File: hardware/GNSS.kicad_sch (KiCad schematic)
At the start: 14 parts, among them J1 Conn_Coaxial, Q1 PMOS, Q2 NMOS, U5 LT6003HDC-TRMPBF, U6 NC7WZ07P6X, U7 NC7WZ07P6X

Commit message: Changes from Reddit review 1
Changed connector, impedance matched the RF traces, changed board to square
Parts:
- J1: footprint Connector_Coaxial:U.FL_Molex_MCRF_73412-0110_Vertical -> Connector_Coaxial:SMA_BAT_Wireless_BWSMA-KWE-Z001
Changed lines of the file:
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@@
 			)
 		)
-		(property "Footprint" "Connector_Coaxial:U.FL_Molex_MCRF_73412-0110_Vertical"
+		(property "Footprint" "Connector_Coaxial:SMA_BAT_Wireless_BWSMA-KWE-Z001"
 			(at 44.45 27.94 0)
 			(effects

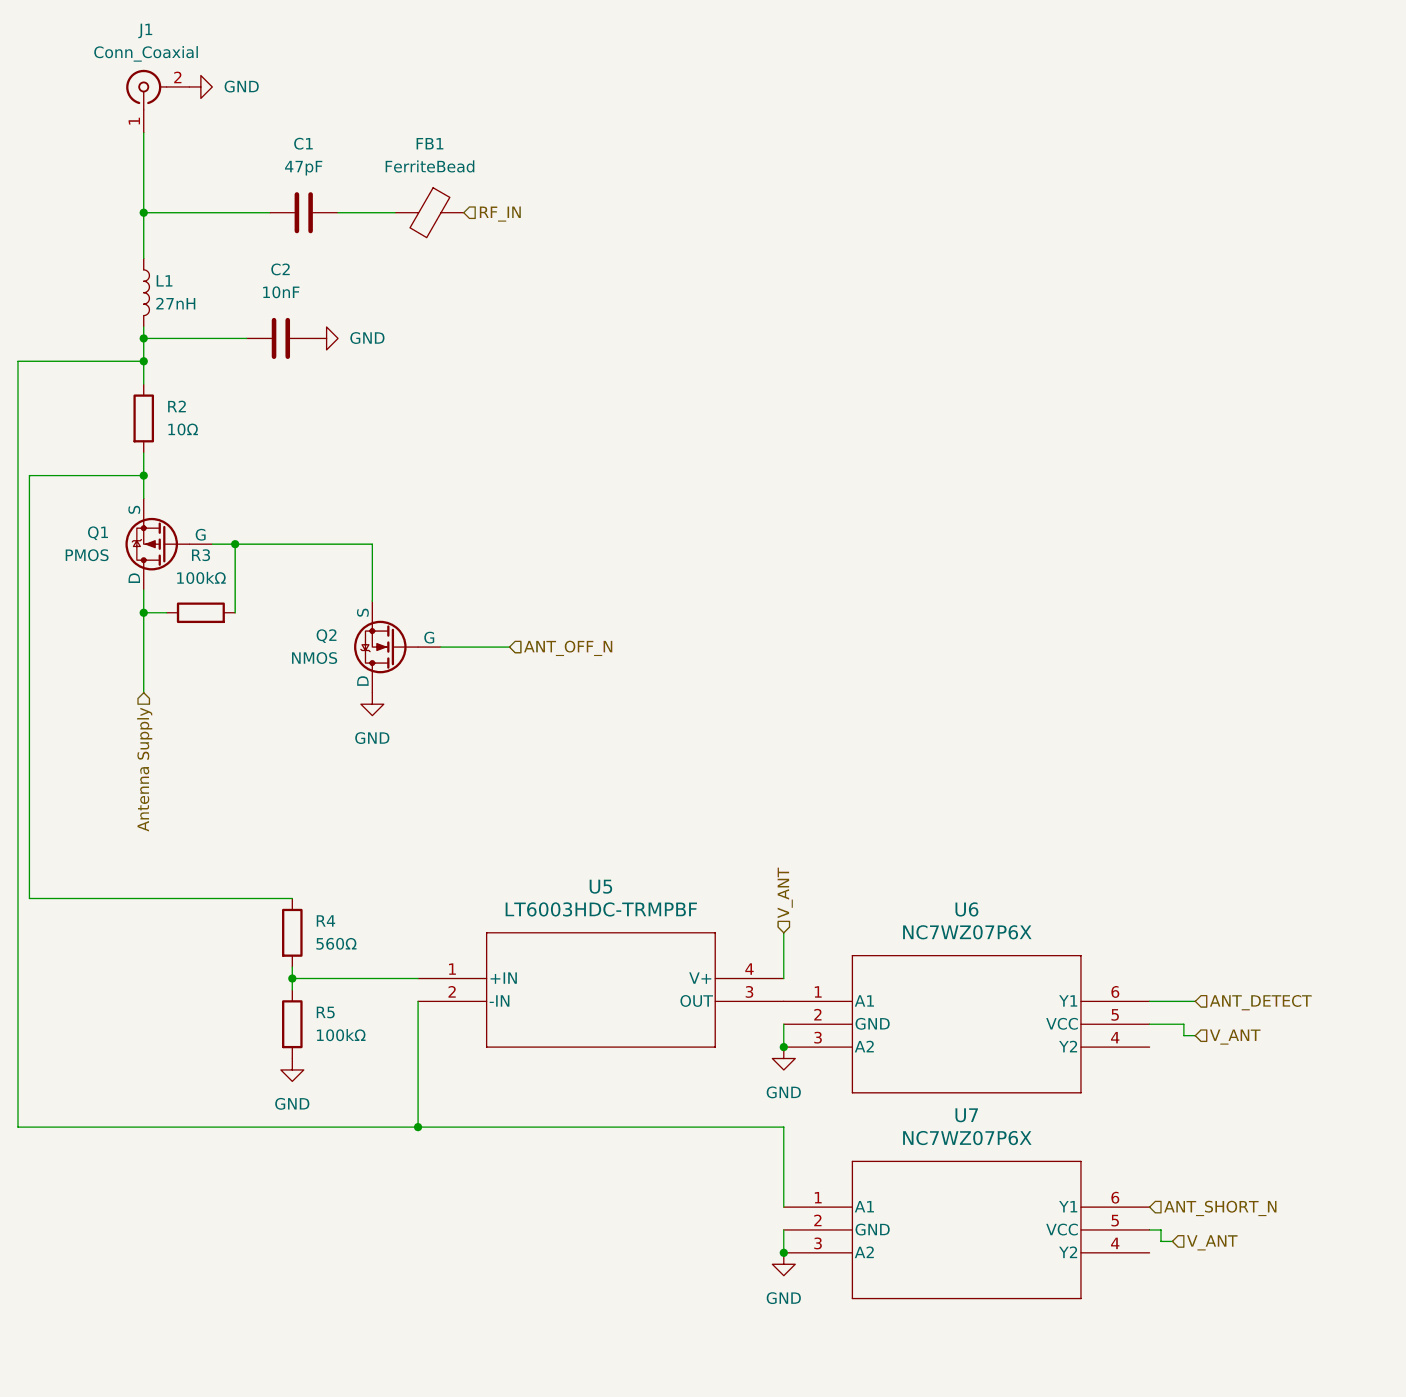
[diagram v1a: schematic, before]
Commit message: many fatal fuck-ups found
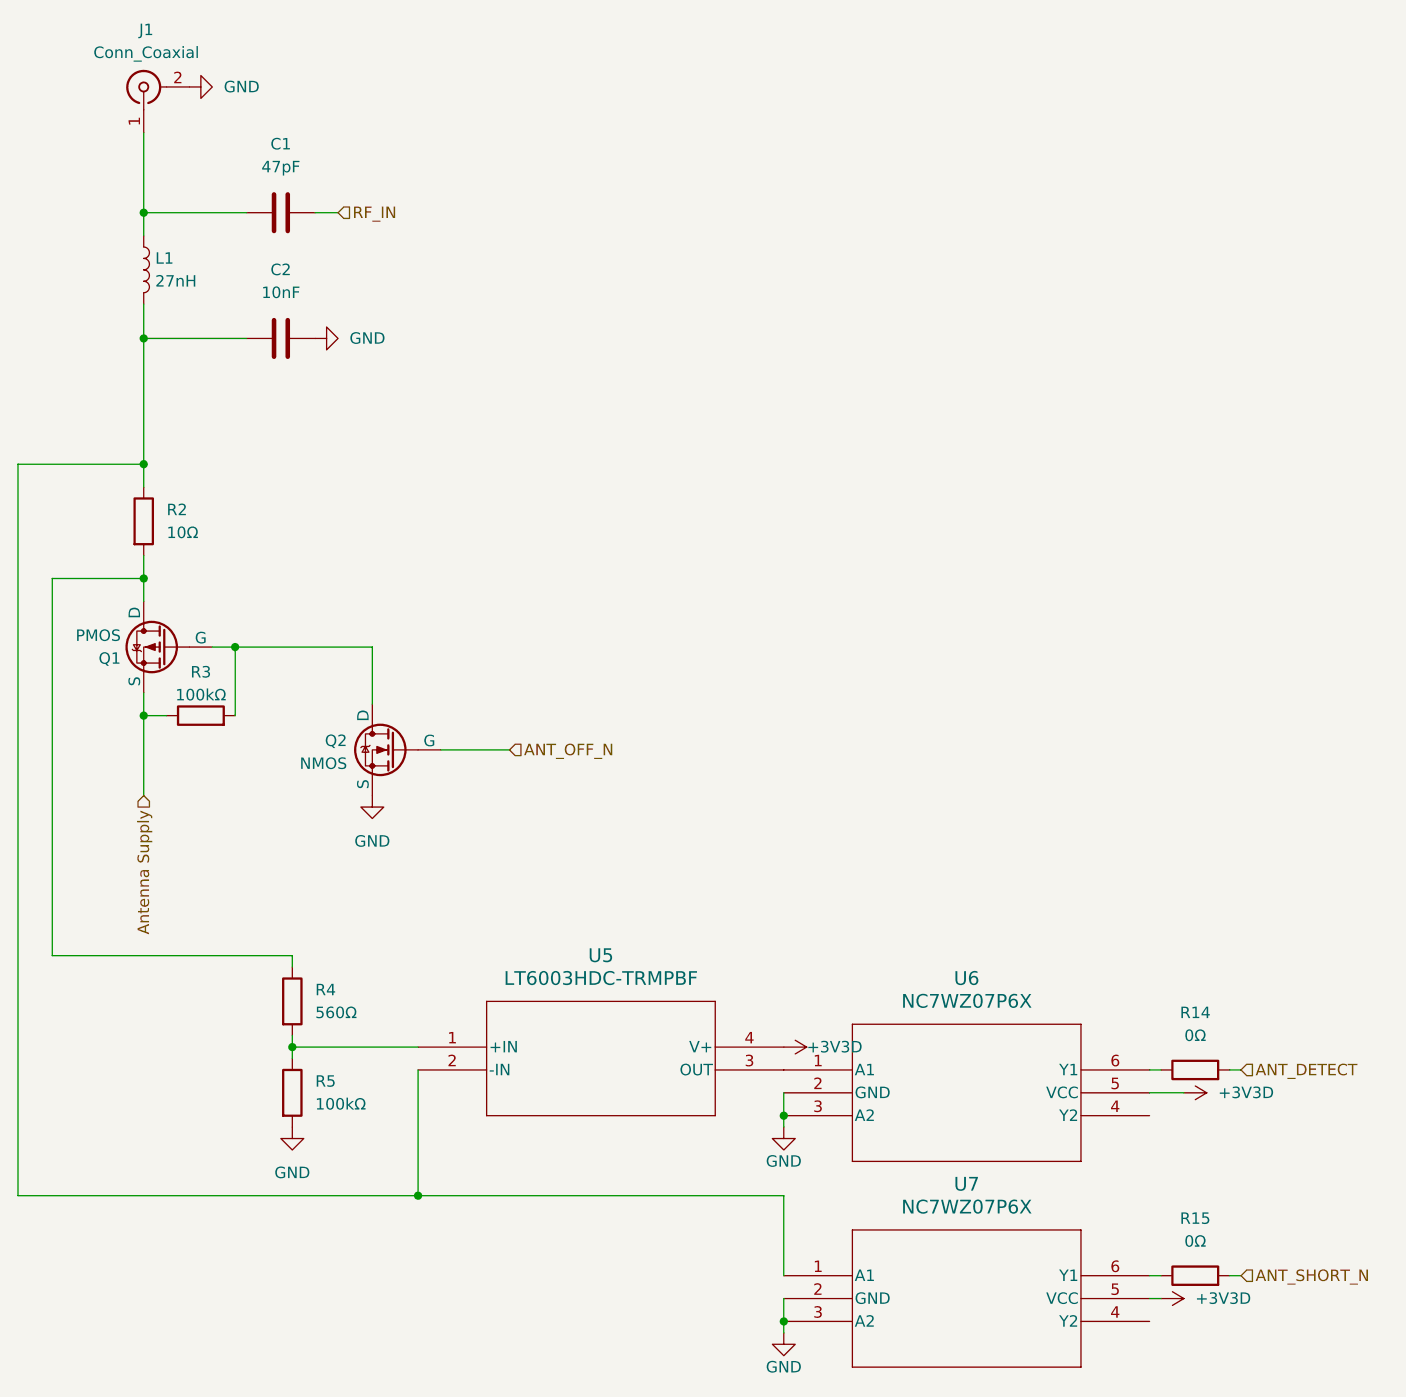
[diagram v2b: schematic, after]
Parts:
- removed FB1: FerriteBead, Capacitor_SMD:C_0402_1005Metric, symbol Device:FerriteBead
- added R14, R15: 0Ω, Resistor_SMD:R_0402_1005Metric, symbol Device:R
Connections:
- net ANT_DETECT: now also R14.2; no longer U6.6 (Y1)
- net ANT_SHORT_N: now also R15.2; no longer U7.6 (Y1)
- net Antenna Supply: now also Q1.3 (S); no longer Q1.1 (D)
- net GND: now also Q2.3 (S); no longer Q2.1 (D)
- net RF_IN: now also C1.2
- net at R2.2, R4.1: now also Q1.1 (D); no longer Q1.3 (S)
- net at Q1.2 (G), R3.2: now also Q2.1 (D); no longer Q2.3 (S)
- net V_ANT renamed +3V3D
- new net: R15.1, U7.6 (Y1)
- new net: R14.1, U6.6 (Y1)
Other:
- moved on the sheet: C1, L1, Q1, Q2, R2, R3, R4, R5, U5, U6, U7
